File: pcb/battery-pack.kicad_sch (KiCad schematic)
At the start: 126 parts, among them Q14 AO3400A, Q15 MMBT5551, Q16 NMOS, Q49 PMOS, U1 BQ76952, U2 LM393, U3 HT7533-1-SOT89

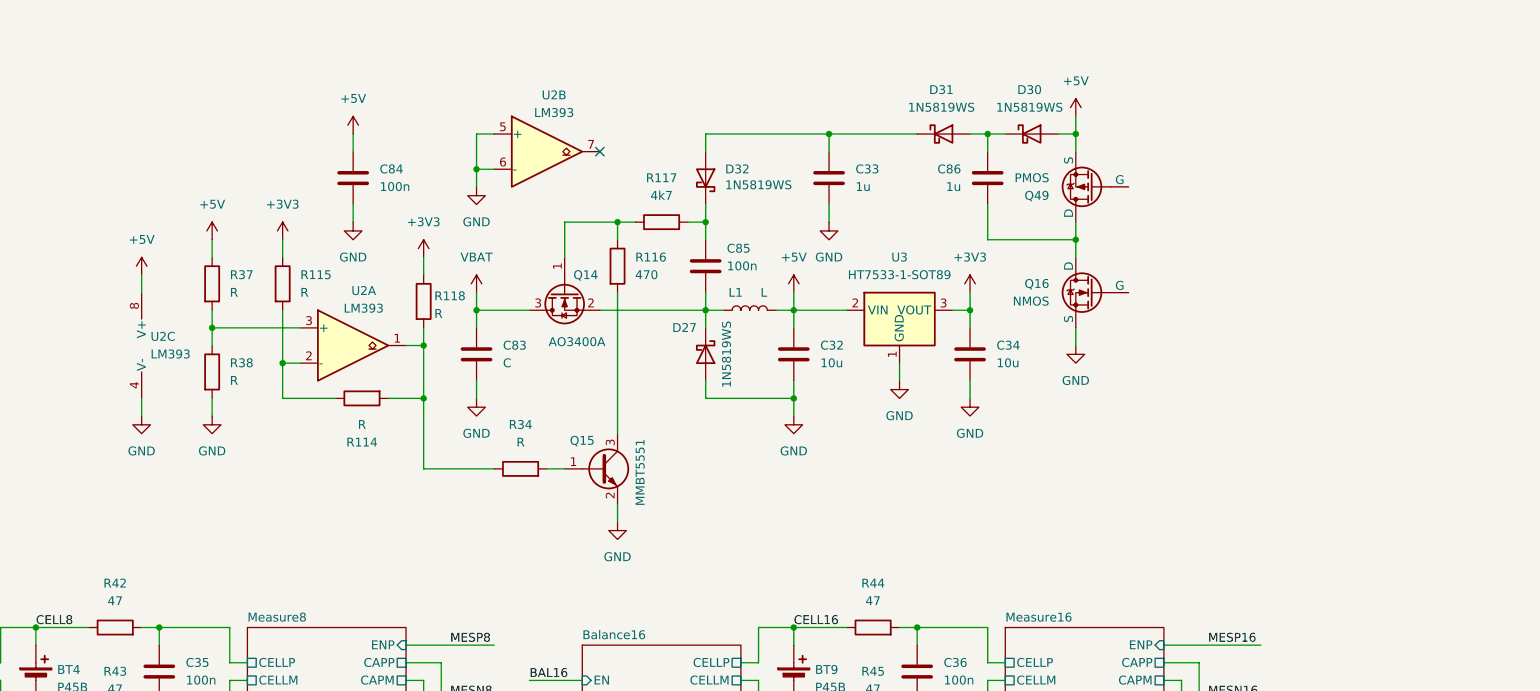
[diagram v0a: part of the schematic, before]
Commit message: Save
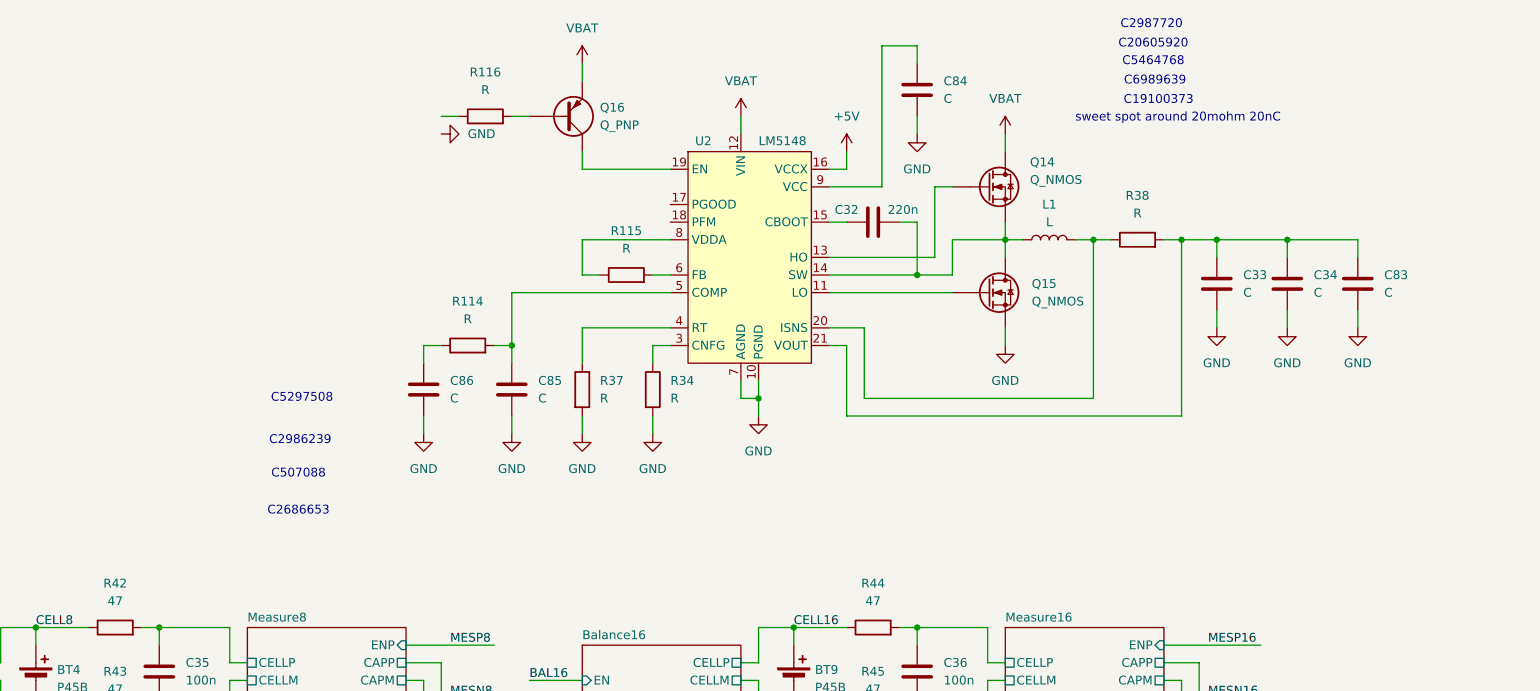
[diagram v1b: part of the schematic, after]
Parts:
- removed D27, D30, D31, D32: 1N5819WS, Diode_SMD:D_SOD-323, symbol Diode:1N5819WS
- removed Q14: AO3400A, Package_TO_SOT_SMD:SOT-23, symbol Transistor_FET:AO3400A
- removed Q15: MMBT5551, Package_TO_SOT_SMD:SOT-23, symbol Transistor_BJT:Q_NPN_BEC
- removed Q16: NMOS, symbol Simulation_SPICE:NMOS
- removed Q49: PMOS, symbol Simulation_SPICE:PMOS
- removed R117: 4k7, symbol Device:R
- removed R118: R, symbol Device:R
- removed U2: LM393, Package_SO:SOIC-8_3.9x4.9mm_P1.27mm, symbol Comparator:LM393
- removed U3: HT7533-1-SOT89, Package_TO_SOT_SMD:SOT-89-3, symbol Regulator_Linear:HT75xx-1-SOT89
- added Q14, Q15: Q_NMOS, symbol Device:Q_NMOS
- added Q16: Q_PNP, symbol Device:Q_PNP
- added U2: LM5148, Package_DFN_QFN:Texas_RGY_R-PVQFN-N24_EP2.05x3.1mm, symbol User_Symbols:LM5148
- C32: value 10u -> 220n; footprint Resistor_SMD:R_0603_1608Metric -> (none); LCSC C19702 -> (none)
- C33, C86: value 1u -> C
- C34: value 10u -> C; footprint Resistor_SMD:R_0603_1608Metric -> (none); LCSC C19702 -> (none)
- C84, C85: value 100n -> C
- R114, R115, R37, R38: footprint Resistor_SMD:R_0402_1005Metric -> (none)
- R116: value 470 -> R
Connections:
- net +5V: now also U2.16 (VCCX); no longer C32.1, C84.1, L1.2, R37.1
- net GND: now also C85.2, C86.2, R34.2, R37.2, Q15.S, U2.1 (NC), U2.10 (PGND), U2.2 (NC), U2.22 (NC), U2.23 (NC), U2.24 (NC), U2.7 (AGND); no longer C32.2, R38.2
- net VBAT: now also Q14.D, Q16.E, U2.12 (VIN); no longer C83.1
- net at C33.1: now also C34.1, C83.1, R38.2, U2.21 (VOUT)
- net at C86.1: now also R114.1
- net at C85.1: now also R114.2, U2.5 (COMP)
- net at L1.1: now also C32.2, Q14.S, Q15.D, U2.14 (SW); no longer C85.2
- net at R34.1: now also U2.3 (CNFG); no longer R114.2
- net at R115.2: now also U2.6 (FB); no longer R114.1
- net at R38.1: now also L1.2, U2.20 (ISNS); no longer R37.2
- net at R116.2: now also Q16.B
- net +3V3: no longer names the net of R115.1
- net +3V3: now also U2.8 (VDDA); no longer C34.1
- new net: Q14.G, U2.13 (HO)
- new net: Q16.C, U2.19 (EN)
- new net: Q15.G, U2.11 (LO)
- new net: C32.1, U2.15 (CBOOT)
- new net: C84.1, U2.9 (VCC)
- new net: R37.1, U2.4 (RT)
- no-connect marks 1 -> 0
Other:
- note added: "C19100373"
- note added: "C20605920"
- note added: "C2686653"
- note added: "C2986239"
- note added: "C2987720"
- note added: "C507088"
- note added: "C5297508"
- note added: "C5464768"
- note added: "C6989639"
- note added: "sweet spot around 20mohm 20nC"
